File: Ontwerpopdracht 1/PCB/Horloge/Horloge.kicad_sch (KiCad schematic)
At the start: 27 parts

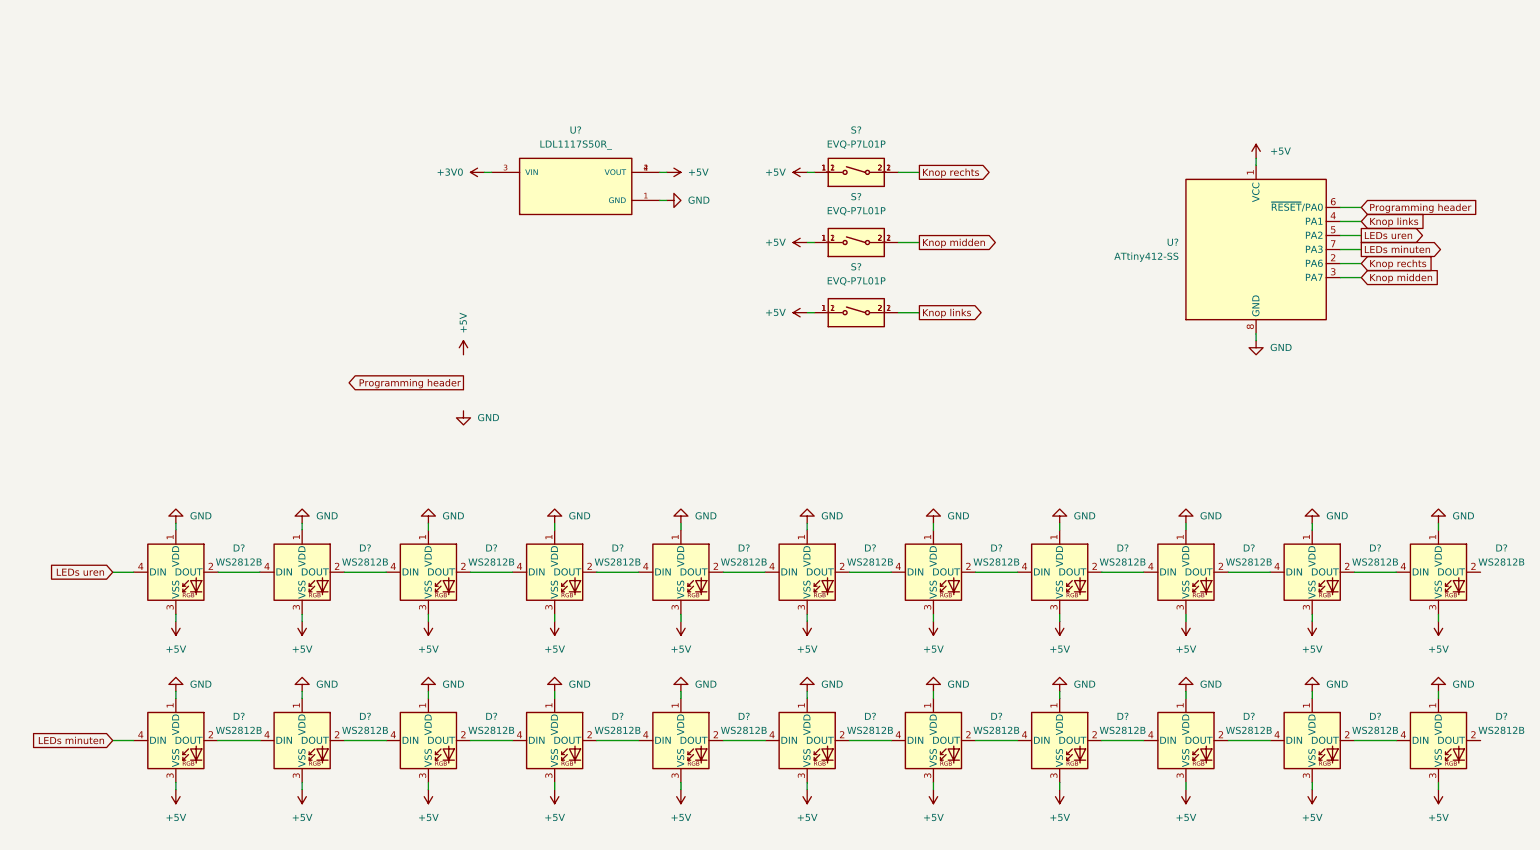
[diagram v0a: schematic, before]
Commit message: schema
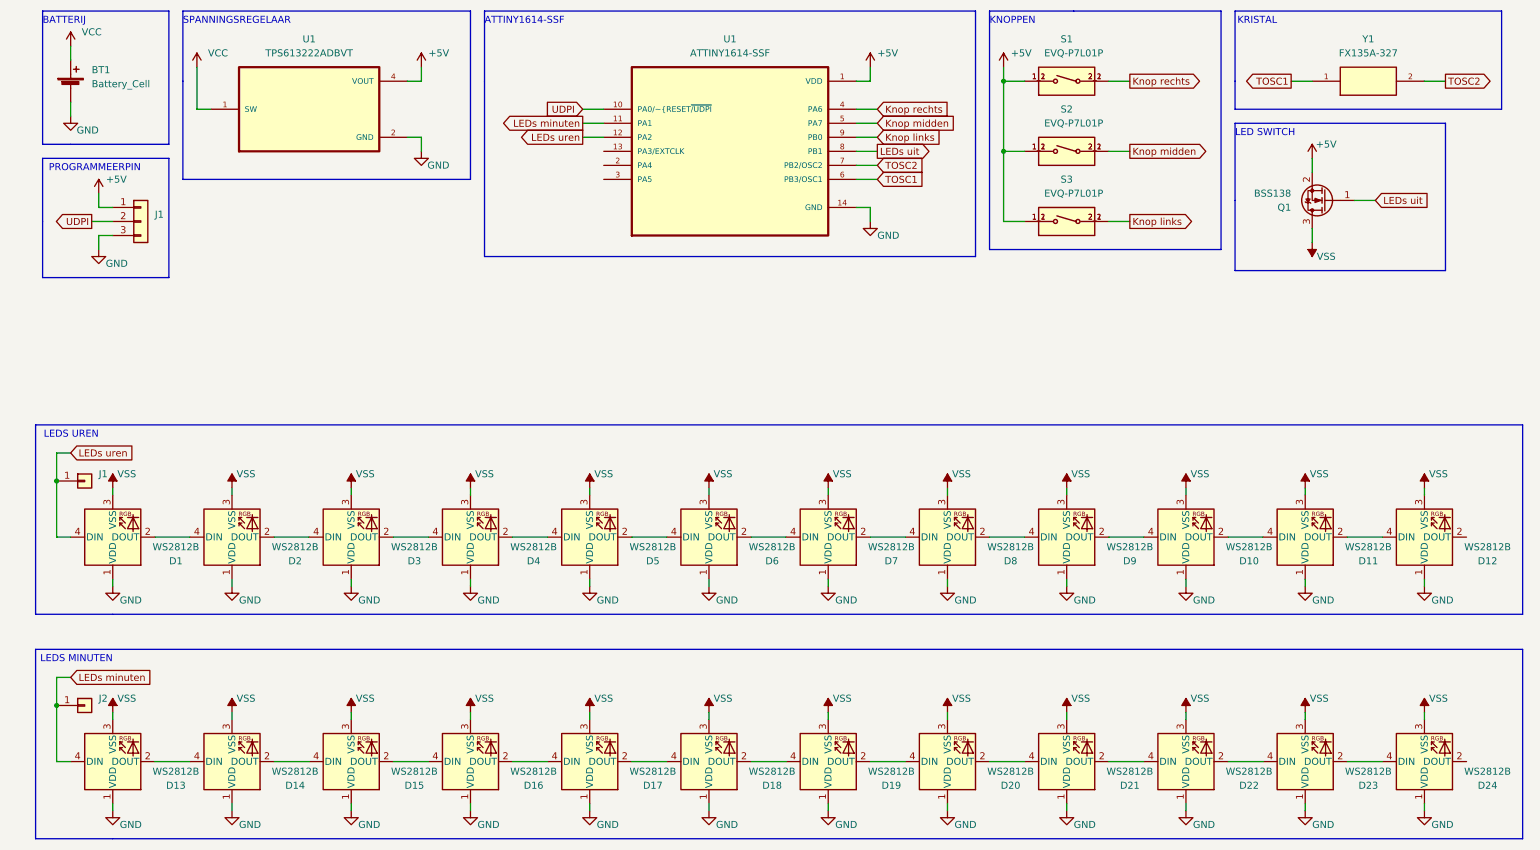
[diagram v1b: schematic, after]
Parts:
- removed D? (x20): WS2812B, LED_SMD:LED_WS2812B_PLCC4_5.0x5.0mm_P3.2mm, symbol LED:WS2812B
- removed U?: LDL1117S50R_, SOT230P700X180-4N, symbol LDL1117S50R_:LDL1117S50R_
- removed U?: ATtiny412-SS, Package_SO:SOIC-8_3.9x4.9mm_P1.27mm, symbol MCU_Microchip_ATtiny:ATtiny412-SS
- added BT1: Battery_Cell, symbol Device:Battery_Cell
- added D10, D11, D12, D13, D14, D15, D16, D17, D18, D19, D20, D21, D22, D23, D24, D3, D4, D5, D6, D7, D8, D9: WS2812B, LED_SMD:LED_WS2812B-2020_PLCC4_2.0x2.0mm, symbol LED:WS2812B
- added J1: Conn_01x03, symbol Connector_Generic:Conn_01x03
- added J1, J2: Conn_01x01, symbol Connector_Generic:Conn_01x01
- added Q1: BSS138, Package_TO_SOT_SMD:SOT-23, symbol Transistor_FET:BSS138
- added U1: TPS613222ADBVT, TPS613222ADBVT:SOT95P280X145-5N, symbol TPS613222ADBVT:TPS613222ADBVT
- added U1: ATTINY1614-SSF, ATTINY1614-SSF:SOIC127P600X175-14N, symbol ATTINY1614-SSF:ATTINY1614-SSF
- added Y1: FX135A-327, FX135A-327:OSCCC150X320X90-2N, symbol FX135A-327:FX135A-327
- D1, D2: renamed from D?; footprint LED_SMD:LED_WS2812B_PLCC4_5.0x5.0mm_P3.2mm -> LED_SMD:LED_WS2812B-2020_PLCC4_2.0x2.0mm
- S1, S2, S3: renamed from S?; footprint SW_EVQ-P7L01P -> EVQ-P7L01P:SW_EVQ-P7L01P
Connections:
- net +5V: now also J1.1 (Pin_1), Q1.2 (S), U1.1 (VDD), U1.4 (VOUT); no longer D1.3 (VSS), D2.3 (VSS)
- net GND: now also BT1.2 (-), D10.1 (VDD), D11.1 (VDD), D12.1 (VDD), D13.1 (VDD), D14.1 (VDD), D15.1 (VDD), D16.1 (VDD), D17.1 (VDD), D18.1 (VDD), D19.1 (VDD), D20.1 (VDD), D21.1 (VDD), D22.1 (VDD), D23.1 (VDD), D24.1 (VDD), D3.1 (VDD), D4.1 (VDD), D5.1 (VDD), D6.1 (VDD), D7.1 (VDD), D8.1 (VDD), D9.1 (VDD), J1.3 (Pin_3), U1.14 (GND), U1.2 (GND)
- net Knop links: now also U1.9 (PB0)
- net Knop midden: now also U1.5 (PA7)
- net Knop rechts: now also U1.4 (PA6)
- net LEDs minuten: now also D13.4 (DIN), J2.1 (Pin_1), U1.11 (PA1)
- net LEDs uren: now also J1.1 (Pin_1), U1.12 (PA2)
- net at D2.2 (DOUT): now also D3.4 (DIN)
- new net: D15.2 (DOUT), D16.4 (DIN)
- new net: D14.2 (DOUT), D15.4 (DIN)
- new net: D13.2 (DOUT), D14.4 (DIN)
- new net: D22.2 (DOUT), D23.4 (DIN)
- new net: D21.2 (DOUT), D22.4 (DIN)
- new net: D6.2 (DOUT), D7.4 (DIN)
- new net: D5.2 (DOUT), D6.4 (DIN)
- new net: D8.2 (DOUT), D9.4 (DIN)
- new net: D7.2 (DOUT), D8.4 (DIN)
- new net: D17.2 (DOUT), D18.4 (DIN)
- new net: D16.2 (DOUT), D17.4 (DIN)
- new net: D23.2 (DOUT), D24.4 (DIN)
- new net: D11.2 (DOUT), D12.4 (DIN)
- new net: D10.2 (DOUT), D11.4 (DIN)
- new net: D10.4 (DIN), D9.2 (DOUT)
- new net: D4.2 (DOUT), D5.4 (DIN)
- new net: D20.2 (DOUT), D21.4 (DIN)
- new net: D19.2 (DOUT), D20.4 (DIN)
- new net: D3.2 (DOUT), D4.4 (DIN)
- new net: D18.2 (DOUT), D19.4 (DIN)
- new net LEDs uit: Q1.1 (G), U1.8 (PB1)
- new net TOSC1: U1.6 (PB3/OSC1), Y1.1
- new net TOSC2: U1.7 (PB2/OSC2), Y1.2
- new net UDPI: J1.2 (Pin_2), U1.10 (PA0/~{RESET~{/UDPI})
- new net VCC: BT1.1 (+), U1.1 (SW)
- new net VSS: D1.3 (VSS), D10.3 (VSS), D11.3 (VSS), D12.3 (VSS), D13.3 (VSS), D14.3 (VSS), D15.3 (VSS), D16.3 (VSS), D17.3 (VSS), D18.3 (VSS), D19.3 (VSS), D2.3 (VSS), D20.3 (VSS), D21.3 (VSS), D22.3 (VSS), D23.3 (VSS), D24.3 (VSS), D3.3 (VSS), D4.3 (VSS), D5.3 (VSS), D6.3 (VSS), D7.3 (VSS), D8.3 (VSS), D9.3 (VSS), Q1.3 (D)
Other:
- note added: "ATTINY1614-SSF"
- note added: "BATTERIJ"
- note added: "KNOPPEN"
- note added: "KRISTAL"
- note added: "LED SWITCH"
- note added: "LEDS MINUTEN"
- note added: "LEDS UREN"
- note added: "PROGRAMMEERPIN"
- note added: "SPANNINGSREGELAAR"
- moved on the sheet: D1, D2, S1, S2, S3
